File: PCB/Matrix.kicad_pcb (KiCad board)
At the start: 2 copper layers, 35.5 x 43.5 mm, 188 parts, among them J1 USB_C_Receptacle_USB2.0_14P, J3 Conn_01x04_Pin, J4 Conn_01x04_Pin, SW1 Switch, U1 RP2040, U2 NCP1117-3.3_SOT223, U3 W25Q128JVS, U4 IS31FL3737, Y1 Crystal_GND24

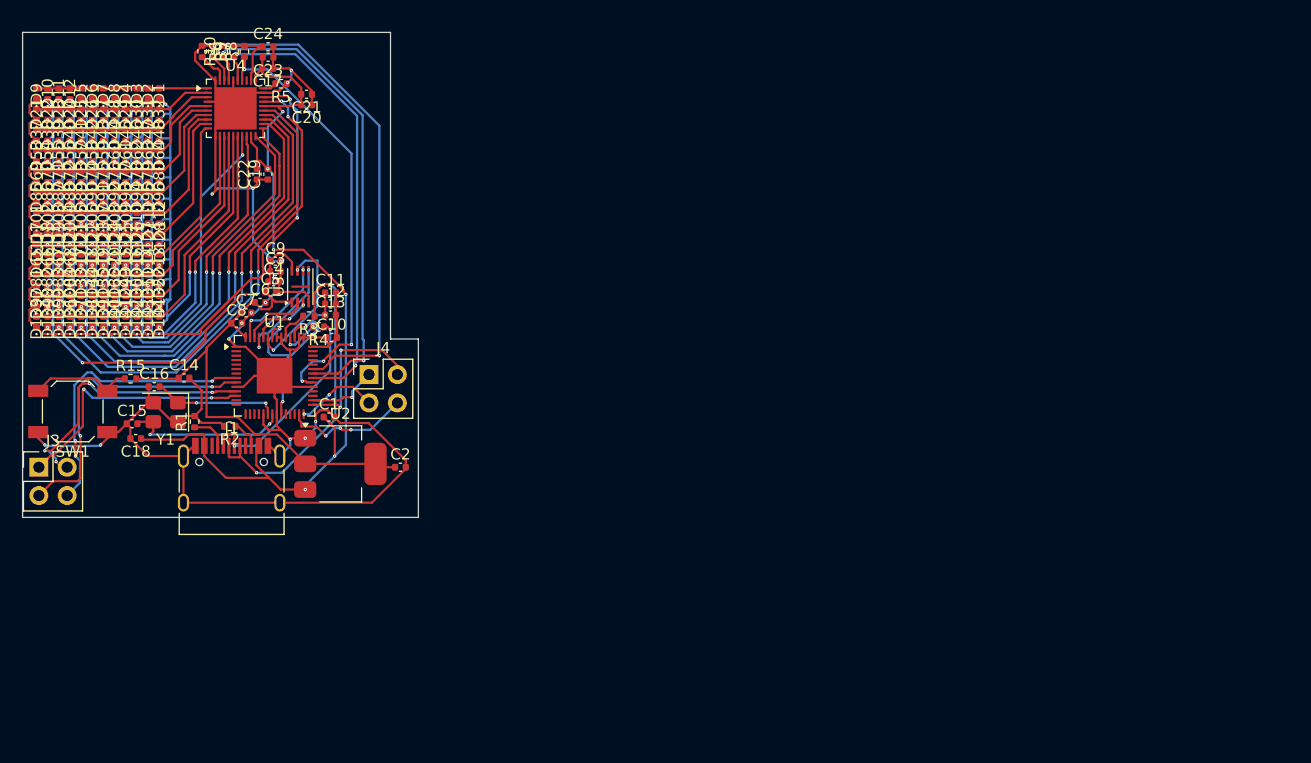
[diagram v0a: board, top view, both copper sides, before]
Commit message: Add files via upload
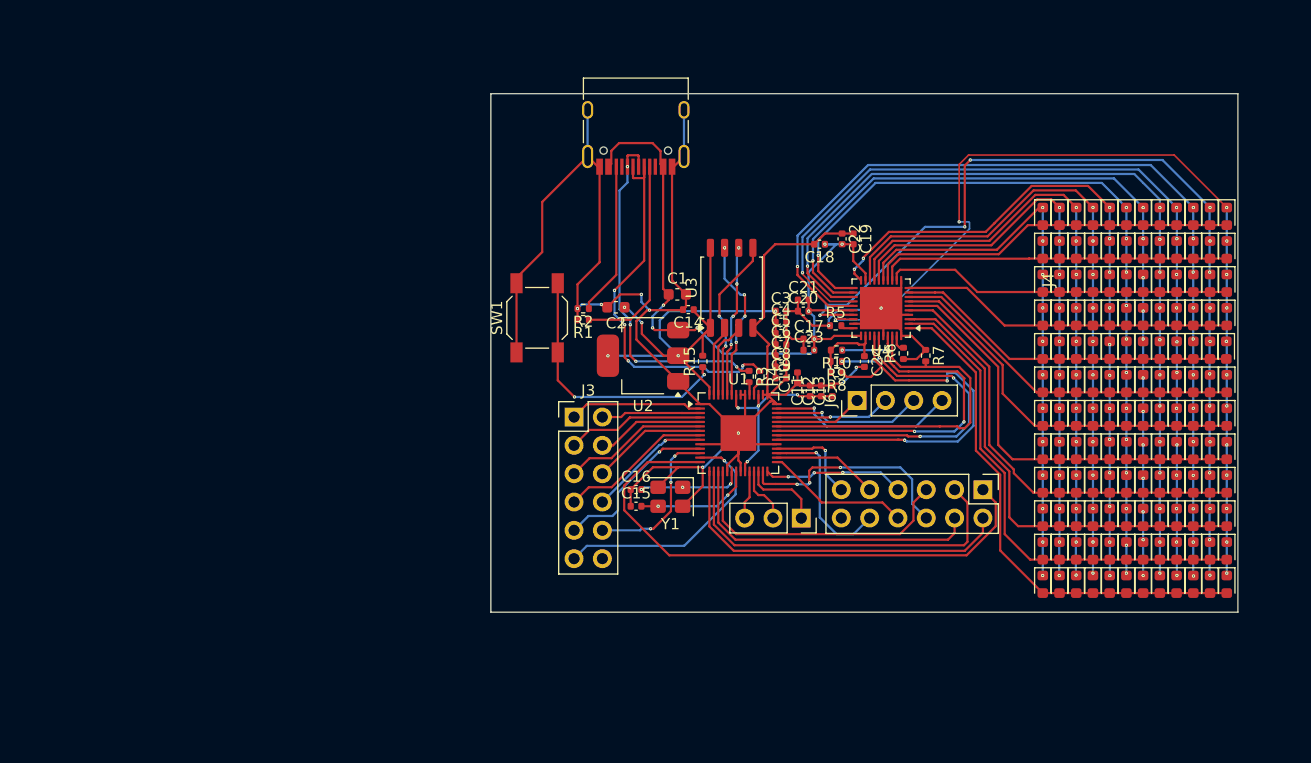
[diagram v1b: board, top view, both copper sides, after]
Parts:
- added J2: Conn_01x03_Pin, Connector_PinSocket_2.54mm:PinSocket_1x03_P2.54mm_Vertical, F.Cu at (234.3, 71.1)
- added J6: Conn_01x04_Socket, Connector_PinHeader_2.54mm:PinHeader_1x04_P2.54mm_Vertical, F.Cu at (239.3, 60.5)
- C1, C2: footprint Capacitor_SMD:C_0402_1005Metric -> Capacitor_SMD:C_0603_1608Metric
- D1, D10, D100, D101, D102, D103, D104, D105, D106, D107, D108, D109, D11, D110, D111, D112, D113, D114, D115, D116, D117, D118, D119, D12, D120, D121, D122, D123, D124, D125, D126, D127, D128, D129, D13, D130, D131, D132, D133, D134, D135, D136, D137, D138, D139, D14, D140, D141, D142, D143, D144, D15, D16, D17, D18, D19, D2, D20, D21, D22, D23, D24, D25, D26, D27, D28, D29, D3, D30, D31, D32, D33, D34, D35, D36, D37, D38, D39, D4, D40, D41, D42, D43, D44, D45, D46, D47, D48, D49, D5, D50, D51, D52, D53, D54, D55, D56, D57, D58, D59, D6, D60, D61, D62, D63, D64, D65, D66, D67, D68, D69, D7, D70, D71, D72, D73, D74, D75, D76, D77, D78, D79, D8, D80, D81, D82, D83, D84, D85, D86, D87, D88, D89, D9, D90, D91, D92, D93, D94, D95, D96, D97, D98, D99: footprint LED_SMD:LED_0402_1005Metric -> LED_SMD:LED_0603_1608Metric
- J3, J4: value Conn_01x04_Pin -> Conn_01x11_Pin; footprint Connector_PinHeader_2.54mm:PinHeader_2x02_P2.54mm_Vertical -> Connector_PinHeader_2.54mm:PinHeader_2x06_P2.54mm_Vertical
- U3: footprint Package_SON:Winbond_USON-8-1EP_3x2mm_P0.5mm_EP0.2x1.6mm -> Package_SO:SOIC-8_5.3x5.3mm_P1.27mm
- moved D9 115.5 mm to (272.5, 77.0), turned to -90 degrees
- moved D21 113.7 mm to (272.5, 74.0), turned to -90 degrees
- moved D10 113.1 mm to (271.0, 77.0), turned to -90 degrees
- moved D37 112.1 mm to (272.5, 71.0), turned to -90 degrees
- moved D22 111.4 mm to (271.0, 74.0), turned to -90 degrees
- moved D11 110.9 mm to (269.5, 77.0), turned to -90 degrees
- moved D53 110.7 mm to (272.5, 68.0), turned to -90 degrees
- moved D38 109.7 mm to (271.0, 71.0), turned to -90 degrees
- moved D69 109.5 mm to (272.5, 65.0), turned to -90 degrees
- moved D23 109.0 mm to (269.5, 74.0), turned to -90 degrees
- moved D12 108.6 mm to (268.0, 77.0), turned to -90 degrees
- moved D85 108.6 mm to (272.5, 62.0), turned to -90 degrees
- moved D54 108.3 mm to (271.0, 68.0), turned to -90 degrees
- moved D101 107.8 mm to (272.5, 59.0), turned to -90 degrees
- moved D39 107.4 mm to (269.5, 71.0), turned to -90 degrees
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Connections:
- U1 pad 11: Net-(J3-Pin_2) -> Net-(J3-Pin_9)
- U1 pad 12: Net-(J3-Pin_1) -> Net-(J3-Pin_10)
- U1 pad 13: unconnected-(U1-GPIO10-Pad13) -> Net-(J3-Pin_11)
- U1 pad 14: unconnected-(U1-GPIO11-Pad14) -> Net-(J4-Pin_1)
- U1 pad 15: unconnected-(U1-GPIO12-Pad15) -> Net-(J4-Pin_2)
- U1 pad 16: unconnected-(U1-GPIO13-Pad16) -> Net-(J4-Pin_3)
- U1 pad 17: unconnected-(U1-GPIO14-Pad17) -> Net-(J4-Pin_4)
- U1 pad 18: unconnected-(U1-GPIO15-Pad18) -> Net-(J4-Pin_5)
- U1 pad 2: unconnected-(U1-GPIO0-Pad2) -> Net-(J3-Pin_1)
- U1 pad 27: Net-(J4-Pin_4) -> Net-(J4-Pin_6)
- U1 pad 28: Net-(J4-Pin_3) -> Net-(J4-Pin_7)
- U1 pad 29: Net-(J4-Pin_2) -> Net-(J4-Pin_8)
- U1 pad 3: unconnected-(U1-GPIO1-Pad3) -> Net-(J3-Pin_2)
- U1 pad 30: Net-(J4-Pin_1) -> Net-(J4-Pin_9)
- U1 pad 31: unconnected-(U1-GPIO20-Pad31) -> Net-(J4-Pin_10)
- U1 pad 32: unconnected-(U1-GPIO21-Pad32) -> Net-(J4-Pin_11)
- U1 pad 38: unconnected-(U1-GPIO26_ADC0-Pad38) -> Net-(J6-Pin_1)
- U1 pad 39: unconnected-(U1-GPIO27_ADC1-Pad39) -> Net-(J6-Pin_2)
- U1 pad 4: unconnected-(U1-GPIO2-Pad4) -> Net-(J3-Pin_3)
- U1 pad 40: unconnected-(U1-GPIO28_ADC2-Pad40) -> Net-(J6-Pin_3)
- U1 pad 41: unconnected-(U1-GPIO29_ADC3-Pad41) -> Net-(J6-Pin_4)
- U1 pad 5: unconnected-(U1-GPIO3-Pad5) -> Net-(J3-Pin_4)
- U1 pad 6: unconnected-(U1-GPIO4-Pad6) -> Net-(J3-Pin_5)
- U1 pad 7: unconnected-(U1-GPIO5-Pad7) -> Net-(J3-Pin_6)
- U1 pad 8: Net-(J3-Pin_4) -> Net-(J3-Pin_7)
- U1 pad 9: Net-(J3-Pin_3) -> Net-(J3-Pin_8)
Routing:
- net Net-(J4-Pin_1): track 6.60 -> 49.7 mm, vias 1 -> 0
- net L1: track 15.4 -> 46.4 mm
- net L2: track 16.0 -> 44.6 mm
- net GND: track 180.7 -> 207.5 mm, vias 15 -> 10
- net Net-(J4-Pin_3): track 7.43 -> 33.6 mm, vias 2 -> 0
- net L3: track 16.6 -> 42.7 mm
- net Net-(J4-Pin_5): track 0.00 -> 25.8 mm
- net Net-(J3-Pin_11): track 0.00 -> 22.6 mm, vias 0 -> 1
- net L4: track 18.2 -> 39.6 mm
- net Net-(J4-Pin_6): track 0.00 -> 20.2 mm, vias 0 -> 3
- net L5: track 19.3 -> 38.3 mm
- net Net-(J4-Pin_2): track 14.2 -> 32.4 mm, vias 2 -> 0
- net Net-(J6-Pin_4): track 0.00 -> 16.8 mm, vias 0 -> 1
- net SDB: track 48.6 -> 31.9 mm, vias 2 -> 0
- net Net-(J4-Pin_4): track 11.5 -> 28.0 mm, vias 3 -> 0
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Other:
- board size 35.5 x 43.5 mm -> 67 x 46.5 mm

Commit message: Add files via upload
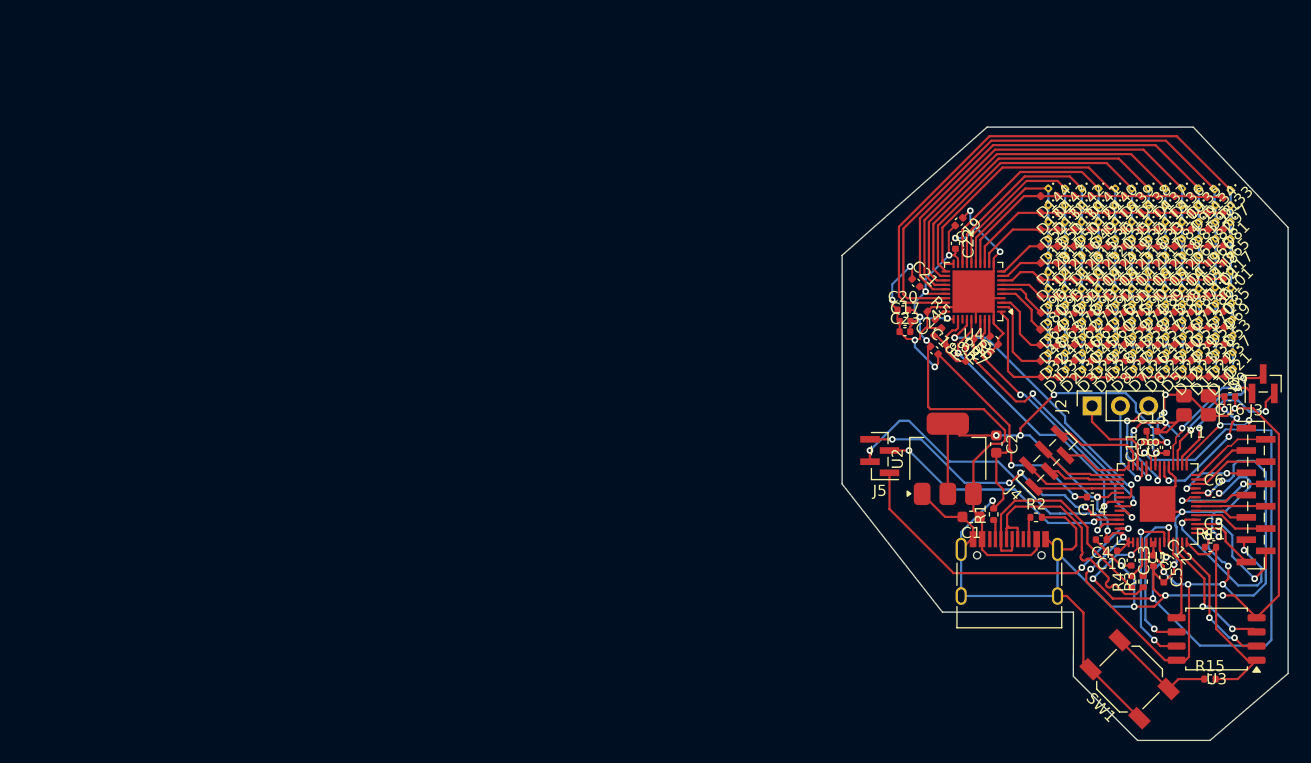
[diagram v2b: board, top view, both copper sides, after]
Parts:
- added J5: Conn_01x04_Pin, Connector_PinHeader_1.00mm:PinHeader_1x04_P1.00mm_Vertical_SMD_Pin1Left, F.Cu at (241.4, 65.5)
- added R11: 10k, Resistor_SMD:R_0402_1005Metric, F.Cu at (271.0, 73.7)
- D1, D10, D100, D101, D102, D103, D104, D105, D106, D107, D108, D109, D11, D110, D111, D112, D113, D114, D115, D116, D117, D118, D119, D12, D120, D121, D122, D123, D124, D125, D126, D127, D128, D129, D13, D130, D131, D132, D133, D134, D135, D136, D137, D138, D139, D14, D140, D141, D142, D143, D144, D15, D16, D17, D18, D19, D2, D20, D21, D22, D23, D24, D25, D26, D27, D28, D29, D3, D30, D31, D32, D33, D34, D35, D36, D37, D38, D39, D4, D40, D41, D42, D43, D44, D45, D46, D47, D48, D49, D5, D50, D51, D52, D53, D54, D55, D56, D57, D58, D59, D6, D60, D61, D62, D63, D64, D65, D66, D67, D68, D69, D7, D70, D71, D72, D73, D74, D75, D76, D77, D78, D79, D8, D80, D81, D82, D83, D84, D85, D86, D87, D88, D89, D9, D90, D91, D92, D93, D94, D95, D96, D97, D98, D99: footprint LED_SMD:LED_0603_1608Metric -> LED_SMD:LED_0402_1005Metric
- J3: value Conn_01x11_Pin -> Conn_01x13_Pin; footprint Connector_PinHeader_2.54mm:PinHeader_2x06_P2.54mm_Vertical -> Connector_PinHeader_1.00mm:PinHeader_1x13_P1.00mm_Vertical_SMD_Pin1Left
- J4: value Conn_01x11_Pin -> Conn_01x06_Pin; footprint Connector_PinHeader_2.54mm:PinHeader_2x06_P2.54mm_Vertical -> Connector_PinHeader_1.00mm:PinHeader_1x06_P1.00mm_Vertical_SMD_Pin1Left
- J6: value Conn_01x04_Socket -> Conn_01x03_Pin; footprint Connector_PinHeader_2.54mm:PinHeader_1x04_P2.54mm_Vertical -> Connector_PinHeader_1.00mm:PinHeader_1x03_P1.00mm_Vertical_SMD_Pin1Left
- moved SW1 62.2 mm to (263.8, 85.5), turned to 135 degrees
- moved J3 61.6 mm to (275.1, 69.0)
- moved C16 53.9 mm to (272.8, 60.2), turned to 180 degrees
- moved U3 53.7 mm to (271.6, 81.9), turned to 180 degrees
- moved R15 53.7 mm to (271.0, 85.5), turned to 0 degrees
- moved J1 53.3 mm to (253.0, 77.0), turned to 0 degrees
- moved Y1 47.9 mm to (269.8, 61.0)
- moved C15 46.8 mm to (265.8, 63.3)
- moved R2 44.7 mm to (255.4, 71.0), turned to 0 degrees
- moved C3 43.8 mm to (271.3, 72.7)
- moved C6 41.0 mm to (271.3, 68.8)
- moved R1 40.7 mm to (251.6, 70.7), turned to 90 degrees
- moved C5 40.7 mm to (266.9, 76.4), turned to -90 degrees
- moved C14 39.9 mm to (260.4, 69.2)
- moved R3 39.8 mm to (265.0, 76.8), turned to 90 degrees
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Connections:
- C10 pad 1: GND -> +3V3
- C14 pad 1: QSPI_SS -> +3V3
- C2 pad 1: QSPI_SS -> +3V3
- C3 pad 1: QSPI_SS -> +3V3
- C4 pad 1: QSPI_SS -> +3V3
- C5 pad 1: QSPI_SS -> +3V3
- C6 pad 1: QSPI_SS -> +3V3
- C7 pad 1: QSPI_SS -> +3V3
- C8 pad 1: QSPI_SS -> +3V3
- C9 pad 1: QSPI_SS -> +3V3
- J3 pad 12: (no net) -> Net-(J3-Pin_12)
- U1 pad 1: GND -> +3V3
- U1 pad 10: GND -> +3V3
- U1 pad 11: Net-(J3-Pin_9) -> Net-(J3-Pin_5)
- U1 pad 12: Net-(J3-Pin_10) -> Net-(J3-Pin_4)
- U1 pad 13: Net-(J3-Pin_11) -> Net-(J3-Pin_3)
- U1 pad 14: Net-(J4-Pin_1) -> Net-(J3-Pin_2)
- U1 pad 15: Net-(J4-Pin_2) -> Net-(J3-Pin_1)
- U1 pad 16: Net-(J4-Pin_3) -> Net-(J6-Pin_3)
- U1 pad 17: Net-(J4-Pin_4) -> Net-(J6-Pin_2)
- U1 pad 18: Net-(J4-Pin_5) -> Net-(J6-Pin_1)
- U1 pad 2: Net-(J3-Pin_1) -> Net-(J3-Pin_13)
- U1 pad 22: GND -> +3V3
- U1 pad 28: Net-(J4-Pin_7) -> Net-(J4-Pin_5)
- U1 pad 29: Net-(J4-Pin_8) -> Net-(J4-Pin_4)
- U1 pad 3: Net-(J3-Pin_2) -> Net-(J3-Pin_12)
- U1 pad 30: Net-(J4-Pin_9) -> Net-(J4-Pin_3)
- U1 pad 31: Net-(J4-Pin_10) -> Net-(J4-Pin_2)
- U1 pad 32: Net-(J4-Pin_11) -> Net-(J4-Pin_1)
- U1 pad 33: GND -> +3V3
- U1 pad 38: Net-(J6-Pin_1) -> Net-(J5-Pin_4)
- U1 pad 39: Net-(J6-Pin_2) -> Net-(J5-Pin_3)
- U1 pad 4: Net-(J3-Pin_3) -> Net-(J3-Pin_11)
- U1 pad 40: Net-(J6-Pin_3) -> Net-(J5-Pin_2)
- U1 pad 41: Net-(J6-Pin_4) -> Net-(J5-Pin_1)
- U1 pad 42: GND -> +3V3
- U1 pad 43: GND -> +3V3
- U1 pad 44: GND -> +3V3
- U1 pad 48: GND -> +3V3
- U1 pad 49: GND -> +3V3
- U1 pad 5: Net-(J3-Pin_4) -> Net-(J3-Pin_10)
- U1 pad 6: Net-(J3-Pin_5) -> Net-(J3-Pin_9)
- U1 pad 7: Net-(J3-Pin_6) -> Net-(J3-Pin_8)
- U1 pad 9: Net-(J3-Pin_8) -> Net-(J3-Pin_6)
- U2 pad 2: QSPI_SS -> +3V3
- U3 pad 8: QSPI_SS -> +3V3
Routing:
- net +3V3: track 0.00 -> 118.3 mm, vias 0 -> 15
- net +1V1: track 17.6 -> 63.2 mm, vias 4 -> 5
- net Net-(J4-Pin_1): track 49.7 -> 7.71 mm
- net QSPI_SS: track 54.9 -> 19.8 mm, vias 5 -> 0
- net C8: track 78.9 -> 47.6 mm, vias 13 -> 0
- net C9: track 81.5 -> 50.6 mm, vias 13 -> 0
- net C7: track 75.1 -> 44.6 mm, vias 13 -> 0
- net C10: track 83.7 -> 53.6 mm, vias 13 -> 0
- net Net-(J5-Pin_2): track 0.00 -> 29.7 mm, vias 0 -> 2
- net C6: track 70.9 -> 41.3 mm, vias 13 -> 0
- net Net-(J5-Pin_1): track 0.00 -> 29.5 mm, vias 0 -> 2
- net Net-(J4-Pin_3): track 33.6 -> 6.55 mm
- net Net-(J5-Pin_4): track 0.00 -> 26.1 mm, vias 0 -> 4
- net C11: track 83.3 -> 59.0 mm, vias 15 -> 0
- net C3: track 55.9 -> 31.8 mm, vias 12 -> 0
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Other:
- board size 67 x 46.5 mm -> 40 x 55 mm
